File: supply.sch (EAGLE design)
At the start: 12 parts

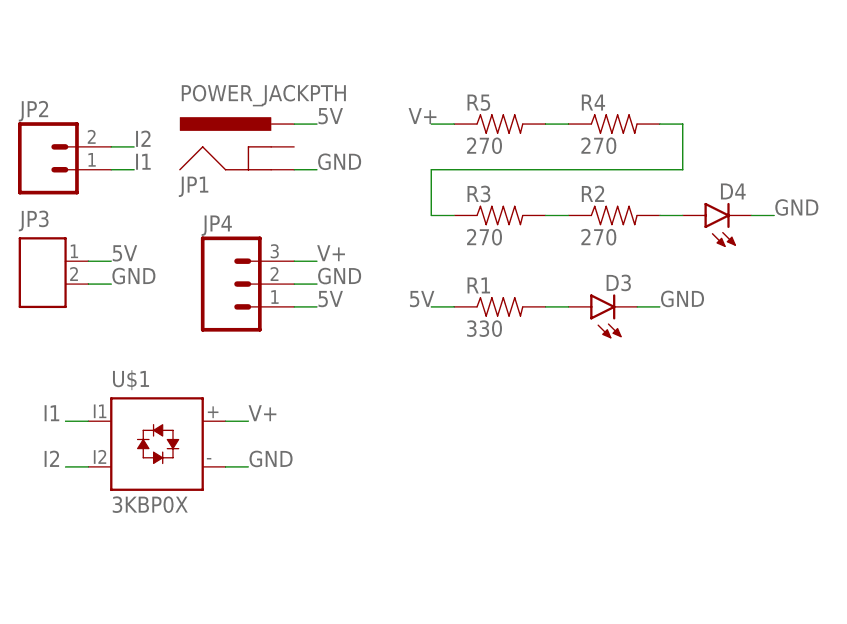
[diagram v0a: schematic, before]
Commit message: update version and documentation
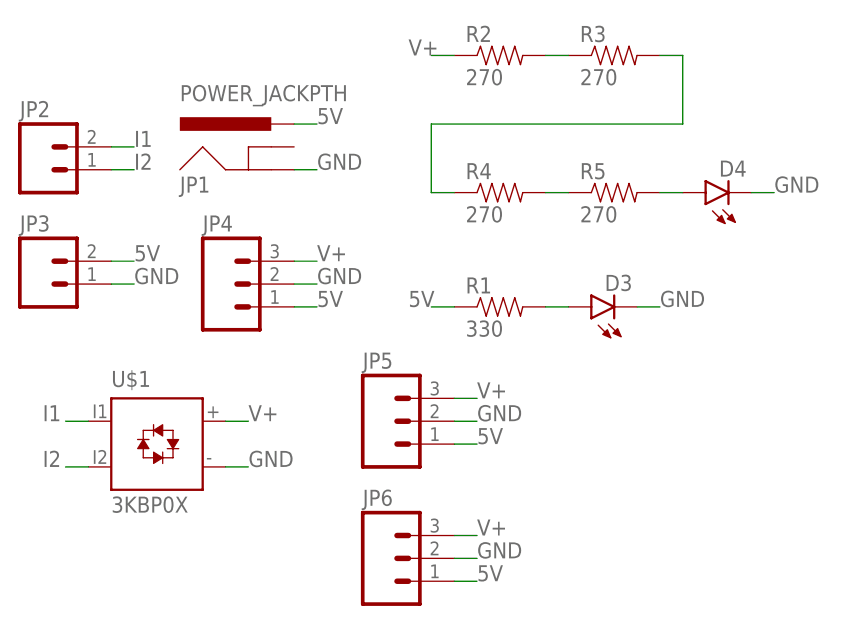
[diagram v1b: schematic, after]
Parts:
- added JP5, JP6: (no value), SparkFun-Connectors:M03PTH
- JP3: value M02 -> (none); device custom-parts:M02 -> SparkFun-Connectors:M02PTH
- JP4: device SparkFun-Connectors:M03LONGPADS -> SparkFun-Connectors:M03PTH
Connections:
- net 5V: now also JP3.2, JP5.1, JP6.1; no longer JP3.P$1
- net GND: now also JP3.1, JP5.2, JP6.2; no longer JP3.P$2
- net I1: now also JP2.2; no longer JP2.1
- net I2: now also JP2.1; no longer JP2.2
- net N$1: now also R2.2, R3.1; no longer R2.1, R3.2
- net N$2: now also D4.A, R5.2; no longer R3.1, R4.2
- net N$3: now also R3.2, R4.1; no longer D4.A, R2.2
- net N$5: now also R4.2, R5.1; no longer R4.1, R5.2
- net V+: now also JP5.3, JP6.3, R2.1; no longer R5.1
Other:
- moved on the sheet: D4, R2, R3, R4, R5
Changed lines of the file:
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@@
 <part name="JP1" library="SparkFun-Connectors" deviceset="POWER_JACK" device="PTH"/>
 <part name="JP2" library="SparkFun-Connectors" deviceset="M02" device="5MM"/>
-<part name="JP3" library="custom-parts" deviceset="M02" device=""/>
 <part name="R1" library="SparkFun-Resistors" deviceset="1KOHM-1/4W-5%(PTH)" device="HORIZ-KIT" value="330"/>
+<part name="R3" library="SparkFun-Resistors" deviceset="1KOHM-1/4W-5%(PTH)" device="HORIZ-KIT" value="270"/>
+<part name="R5" library="SparkFun-Resistors" deviceset="1KOHM-1/4W-5%(PTH)" device="HORIZ-KIT" value="270"/>
+<part name="R4" library="SparkFun-Resistors" deviceset="1KOHM-1/4W-5%(PTH)" device="HORIZ-KIT" value="270"/>
 <part name="R2" library="SparkFun-Resistors" deviceset="1KOHM-1/4W-5%(PTH)" device="HORIZ-KIT" value="270"/>
-<part name="R4" library="SparkFun-Resistors" deviceset="1KOHM-1/4W-5%(PTH)" device="HORIZ-KIT" value="270"/>
-<part name="R5" library="SparkFun-Resistors" deviceset="1KOHM-1/4W-5%(PTH)" device="HORIZ-KIT" value="270"/>
-<part name="R3" library="SparkFun-Resistors" deviceset="1KOHM-1/4W-5%(PTH)" device="HORIZ-KIT" value="270"/>
 <part name="D3" library="SparkFun-LED" deviceset="LED" device="10MM"/>
 <part name="D4" library="SparkFun-LED" deviceset="LED" device="10MM"/>
-<part name="JP4" library="SparkFun-Connectors" deviceset="M03" device="LONGPADS"/>
+<part name="JP4" library="SparkFun-Connectors" deviceset="M03" device="PTH"/>
+<part name="JP3" library="SparkFun-Connectors" deviceset="M02" device="PTH"/>
+<part name="JP5" library="SparkFun-Connectors" deviceset="M03" device="PTH"/>
+<part name="JP6" library="SparkFun-Connectors" deviceset="M03" device="PTH"/>
 </parts>
 <sheets>
@@
 <instance part="JP1" gate="G$1" x="25.4" y="35.56"/>
 <instance part="JP2" gate="G$1" x="0" y="38.1"/>
+<instance part="R1" gate="G$1" x="50.8" y="22.86"/>
+<instance part="R3" gate="G$1" x="63.5" y="50.8"/>
+<instance part="R5" gate="G$1" x="63.5" y="35.56"/>
+<instance part="R4" gate="G$1" x="50.8" y="35.56"/>
+<instance part="R2" gate="G$1" x="50.8" y="50.8"/>
+<instance part="D3" gate="G$1" x="60.96" y="22.86" rot="R90"/>
+<instance part="D4" gate="G$1" x="73.66" y="35.56" rot="R90"/>
+<instance part="JP4" gate="G$1" x="20.32" y="25.4"/>
 <instance part="JP3" gate="G$1" x="0" y="25.4"/>
-<instance part="R1" gate="G$1" x="50.8" y="22.86"/>
-<instance part="R2" gate="G$1" x="63.5" y="33.02"/>
-<instance part="R4" gate="G$1" x="63.5" y="43.18"/>
-<instance part="R5" gate="G$1" x="50.8" y="43.18"/>
-<instance part="R3" gate="G$1" x="50.8" y="33.02"/>
-<instance part="D3" gate="G$1" x="60.96" y="22.86" rot="R90"/>
-<instance part="D4" gate="G$1" x="73.66" y="33.02" rot="R90"/>
-<instance part="JP4" gate="G$1" x="20.32" y="25.4"/>
+<instance part="JP5" gate="G$1" x="38.1" y="10.16"/>
+<instance part="JP6" gate="G$1" x="38.1" y="-5.08"/>
 </instances>
 <busses>
@@
 </segment>
 <segment>
+<pinref part="JP2" gate="G$1" pin="2"/>
+<wire x1="7.62" y1="40.64" x2="10.16" y2="40.64" width="0.1524" layer="91"/>
+<label x="10.16" y="40.64" size="1.778" layer="95"/>
+</segment>
+</net>
+<net name="I2" class="0">
+<segment>
+<pinref part="U$1" gate="G$1" pin="I2"/>
+<wire x1="5.08" y1="5.08" x2="2.54" y2="5.08" width="0.1524" layer="91"/>
+<label x="0" y="5.08" size="1.778" layer="95"/>
+</segment>
+<segment>
 <pinref part="JP2" gate="G$1" pin="1"/>
 <wire x1="7.62" y1="38.1" x2="10.16" y2="38.1" width="0.1524" layer="91"/>
@@
 </segment>
 </net>
-<net name="I2" class="0">
-<segment>
-<pinref part="U$1" gate="G$1" pin="I2"/>
-<wire x1="5.08" y1="5.08" x2="2.54" y2="5.08" width="0.1524" layer="91"/>
-<label x="0" y="5.08" size="1.778" layer="95"/>
-</segment>
-<segment>
-<pinref part="JP2" gate="G$1" pin="2"/>
-<wire x1="7.62" y1="40.64" x2="10.16" y2="40.64" width="0.1524" layer="91"/>
-<label x="10.16" y="40.64" size="1.778" layer="95"/>
-</segment>
-</net>
 <net name="5V" class="0">
 <segment>
@@
 </segment>
 <segment>
-<pinref part="JP3" gate="G$1" pin="P$1"/>
-<wire x1="5.08" y1="27.94" x2="7.62" y2="27.94" width="0.1524" layer="91"/>
-<label x="7.62" y="27.94" size="1.778" layer="95"/>
+<wire x1="7.62" y1="27.94" x2="10.16" y2="27.94" width="0.1524" layer="91"/>
+<label x="10.16" y="27.94" size="1.778" layer="95"/>
+<pinref part="JP3" gate="G$1" pin="2"/>
 </segment>
 <segment>
@@
 <pinref part="JP4" gate="G$1" pin="1"/>
 </segment>
+<segment>
+<wire x1="45.72" y1="7.62" x2="48.26" y2="7.62" width="0.1524" layer="91"/>
+<label x="48.26" y="7.62" size="1.778" layer="95"/>
+<pinref part="JP5" gate="G$1" pin="1"/>
+</segment>
+<segment>
+<wire x1="45.72" y1="-7.62" x2="48.26" y2="-7.62" width="0.1524" layer="91"/>
+<label x="48.26" y="-7.62" size="1.778" layer="95"/>
+<pinref part="JP6" gate="G$1" pin="1"/>
+</segment>
 </net>
 <net name="GND" class="0">
@@
 </segment>
 <segment>
-<pinref part="JP3" gate="G$1" pin="P$2"/>
-<wire x1="5.08" y1="25.4" x2="7.62" y2="25.4" width="0.1524" layer="91"/>
-<label x="7.62" y="25.4" size="1.778" layer="95"/>
+<wire x1="7.62" y1="25.4" x2="10.16" y2="25.4" width="0.1524" layer="91"/>
+<label x="10.16" y="25.4" size="1.778" layer="95"/>
+<pinref part="JP3" gate="G$1" pin="1"/>
 </segment>
 <segment>
@@
 </segment>
 <segment>
-<wire x1="78.74" y1="33.02" x2="81.28" y2="33.02" width="0.1524" layer="91"/>
-<label x="81.28" y="33.02" size="1.778" layer="95"/>
+<wire x1="78.74" y1="35.56" x2="81.28" y2="35.56" width="0.1524" layer="91"/>
+<label x="81.28" y="35.56" size="1.778" layer="95"/>
 <pinref part="D4" gate="G$1" pin="C"/>
 </segment>
@@
 <pinref part="JP4" gate="G$1" pin="2"/>
 </segment>
+<segment>
+<wire x1="45.72" y1="10.16" x2="48.26" y2="10.16" width="0.1524" layer="91"/>
+<label x="48.26" y="10.16" size="1.778" layer="95"/>
+<pinref part="JP5" gate="G$1" pin="2"/>
+</segment>
+<segment>
+<wire x1="45.72" y1="-5.08" x2="48.26" y2="-5.08" width="0.1524" layer="91"/>
+<label x="48.26" y="-5.08" size="1.778" layer="95"/>
+<pinref part="JP6" gate="G$1" pin="2"/>
+</segment>
 </net>
 <net name="V+" class="0">
-<segment>
-<pinref part="R5" gate="G$1" pin="1"/>
-<wire x1="45.72" y1="43.18" x2="43.18" y2="43.18" width="0.1524" layer="91"/>
-<label x="40.64" y="43.18" size="1.778" layer="95"/>
-</segment>
 <segment>
 <pinref part="U$1" gate="G$1" pin="+"/>
@@
 <pinref part="JP4" gate="G$1" pin="3"/>
 </segment>
-</net>
-<net name="N$3" class="0">
-<segment>
-<pinref part="R2" gate="G$1" pin="2"/>
-<wire x1="68.58" y1="33.02" x2="71.12" y2="33.02" width="0.1524" layer="91"/>
-<pinref part="D4" gate="G$1" pin="A"/>
+<segment>
+<pinref part="R2" gate="G$1" pin="1"/>
+<wire x1="45.72" y1="50.8" x2="43.18" y2="50.8" width="0.1524" layer="91"/>
+<label x="40.64" y="50.8" size="1.778" layer="95"/>
+</segment>
+<segment>
+<wire x1="45.72" y1="12.7" x2="48.26" y2="12.7" width="0.1524" layer="91"/>
+<label x="48.26" y="12.7" size="1.778" layer="95"/>
+<pinref part="JP5" gate="G$1" pin="3"/>
+</segment>
+<segment>
+<wire x1="45.72" y1="-2.54" x2="48.26" y2="-2.54" width="0.1524" layer="91"/>
+<label x="48.26" y="-2.54" size="1.778" layer="95"/>
+<pinref part="JP6" gate="G$1" pin="3"/>
 </segment>
 </net>
@@
 <net name="N$1" class="0">
 <segment>
-<pinref part="R2" gate="G$1" pin="1"/>
+<pinref part="R3" gate="G$1" pin="1"/>
+<pinref part="R2" gate="G$1" pin="2"/>
+<wire x1="58.42" y1="50.8" x2="55.88" y2="50.8" width="0.1524" layer="91"/>
+</segment>
+</net>
+<net name="N$2" class="0">
+<segment>
+<pinref part="R5" gate="G$1" pin="2"/>
+<wire x1="71.12" y1="35.56" x2="68.58" y2="35.56" width="0.1524" layer="91"/>
+<pinref part="D4" gate="G$1" pin="A"/>
+</segment>
+</net>
+<net name="N$5" class="0">
+<segment>
+<pinref part="R4" gate="G$1" pin="2"/>
+<pinref part="R5" gate="G$1" pin="1"/>
+<wire x1="55.88" y1="35.56" x2="58.42" y2="35.56" width="0.1524" layer="91"/>
+</segment>
+</net>
+<net name="N$3" class="0">
+<segment>
+<pinref part="R4" gate="G$1" pin="1"/>
+<wire x1="45.72" y1="35.56" x2="43.18" y2="35.56" width="0.1524" layer="91"/>
+<wire x1="43.18" y1="35.56" x2="43.18" y2="43.18" width="0.1524" layer="91"/>
+<wire x1="43.18" y1="43.18" x2="71.12" y2="43.18" width="0.1524" layer="91"/>
+<wire x1="71.12" y1="43.18" x2="71.12" y2="50.8" width="0.1524" layer="91"/>
 <pinref part="R3" gate="G$1" pin="2"/>
-<wire x1="58.42" y1="33.02" x2="55.88" y2="33.02" width="0.1524" layer="91"/>
-</segment>
-</net>
-<net name="N$2" class="0">
-<segment>
-<pinref part="R3" gate="G$1" pin="1"/>
-<wire x1="45.72" y1="33.02" x2="43.18" y2="33.02" width="0.1524" layer="91"/>
-<wire x1="43.18" y1="33.02" x2="43.18" y2="38.1" width="0.1524" layer="91"/>
-<wire x1="43.18" y1="38.1" x2="71.12" y2="38.1" width="0.1524" layer="91"/>
-<wire x1="71.12" y1="38.1" x2="71.12" y2="43.18" width="0.1524" layer="91"/>
-<pinref part="R4" gate="G$1" pin="2"/>
-<wire x1="71.12" y1="43.18" x2="68.58" y2="43.18" width="0.1524" layer="91"/>
-</segment>
-</net>
-<net name="N$5" class="0">
-<segment>
-<pinref part="R5" gate="G$1" pin="2"/>
-<pinref part="R4" gate="G$1" pin="1"/>
-<wire x1="55.88" y1="43.18" x2="58.42" y2="43.18" width="0.1524" layer="91"/>
-</segment>
-</net>
+<wire x1="71.12" y1="50.8" x2="68.58" y2="50.8" width="0.1524" layer="91"/>
+</segment>
+</net>
